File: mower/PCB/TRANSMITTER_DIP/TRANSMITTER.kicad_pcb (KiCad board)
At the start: 2 copper layers, 55 x 41.6 mm, 14 parts, among them J1 BOT POWER, J2 POWER IN, J3 SHUNT, J4 COIL OUT, J5 COIL POWER IN, Q1 IRF3205, U1 LM358, U4 LM555xN

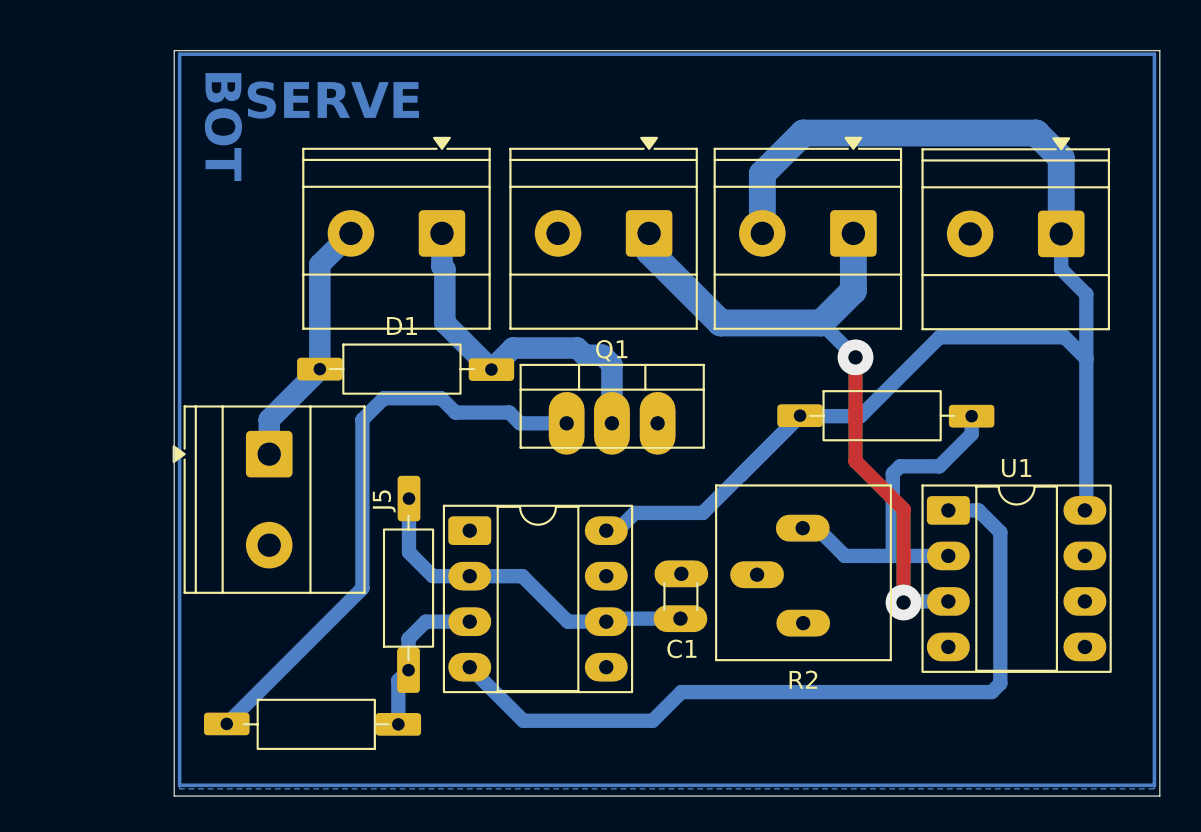
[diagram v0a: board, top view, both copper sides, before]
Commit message: .
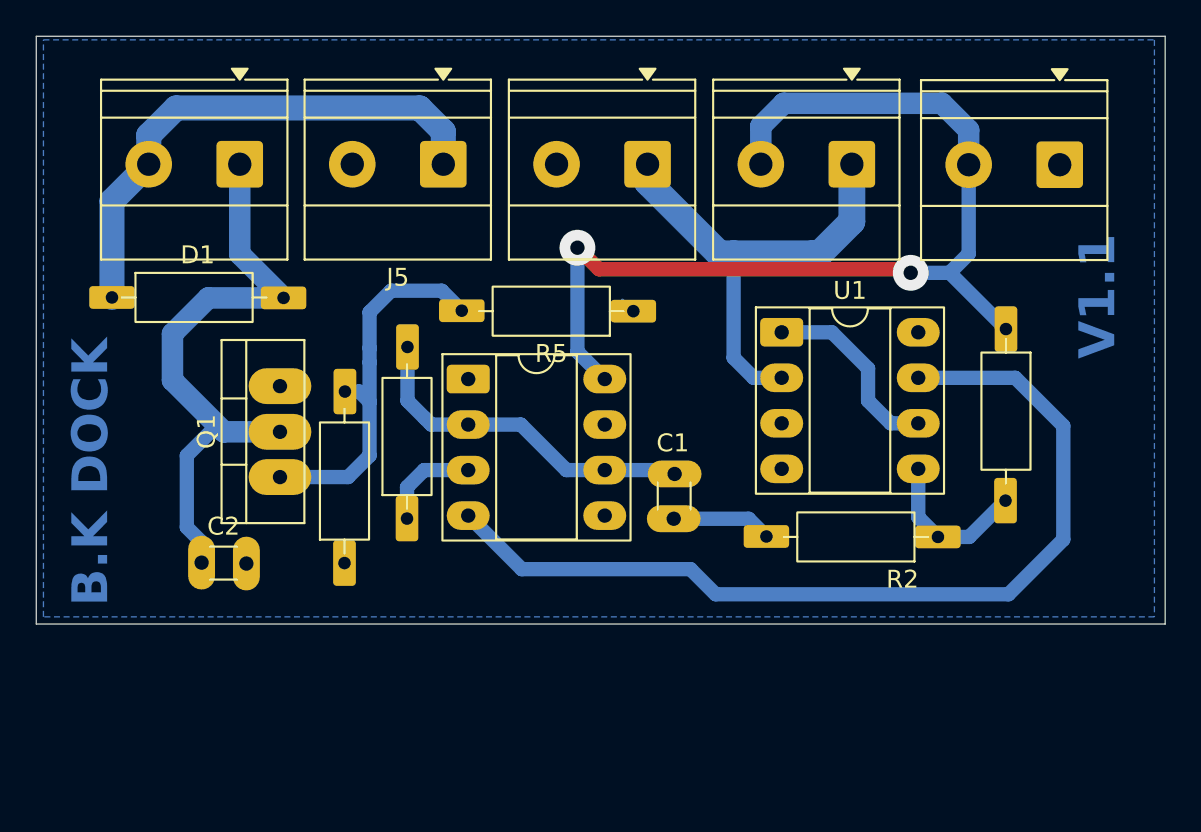
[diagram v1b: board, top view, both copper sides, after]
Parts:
- added C2: 100nF, IMRANS_LIBRARY:C_Disc_D3.0mm_W1.6mm_P2.50mm, F.Cu at (104.0, 63.6)
- added R5: 1K, IMRANS_LIBRARY:R_Axial_DIN0207_L6.3mm_D2.5mm_P10.16mm_Horizontal_2, F.Cu at (128.6, 49.5)
- D1: value 1N5819 -> 1N4007
- R1: value 10k -> 10K
- R2: value 10k -> 10K; footprint IMRANS_LIBRARY:Potentiometer_Bourns_3386P_Vertical -> IMRANS_LIBRARY:R_Axial_DIN0207_L6.3mm_D2.5mm_P10.16mm_Horizontal_2
- moved J5 18.9 mm to (117.5, 41.3), turned to 180 degrees
- moved Q1 16.3 mm to (108.4, 58.8), turned to 90 degrees
- moved U1 13.6 mm to (136.4, 50.7)
- moved R1 13.1 mm to (148.9, 50.0), turned to -90 degrees
- moved D1 12.3 mm to (98.5, 48.8)
- moved J4 11.9 mm to (106.2, 41.3)
- moved R4 9.19 mm to (112.0, 64.1), turned to 90 degrees
- moved R3 8.46 mm to (115.5, 61.6)
- moved U4 8.46 mm to (118.9, 53.3)
- moved C1 8.13 mm to (130.4, 58.6), turned to -90 degrees
- moved R2 8.04 mm to (145.6, 62.1)
- moved J1 3.86 mm to (128.9, 41.3)
- moved J2 3.86 mm to (151.9, 41.4)
- moved J3 3.86 mm to (140.3, 41.3)
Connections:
- J2 pad 1: VCC -> GND
- J2 pad 2: GND -> VCC
- R1 pad 2: Net-(U1A--) -> Net-(U1B-+)
- R2 pad 1: Net-(U1A--) -> Net-(U1B-+)
- U1 pad 1: Net-(U4-R) -> Net-(U1B--)
- U1 pad 2: Net-(U1A--) -> Net-(J1-Pin_1)
- U1 pad 3: Net-(J1-Pin_1) -> GND
- U1 pad 4: GND -> unconnected-(U1C-V--Pad4)
- U1 pad 5: (no net) -> Net-(U1B-+)
- U1 pad 6: (no net) -> Net-(U1B--)
- U1 pad 7: (no net) -> Net-(U4-R)
- U1 pad 8: VCC -> unconnected-(U1C-V+-Pad8)
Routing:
- net VCC: track 79.1 -> 57.0 mm, vias 0 -> 2
- net Net-(U1A--): track 18.9 -> 0.00 mm
- net VCOIL: track 14.2 -> 29.3 mm
- net Net-(D1-A): track 20.3 -> 34.2 mm
- net Net-(Q1-G): track 34.0 -> 21.2 mm
- net Net-(J1-Pin_1): track 38.0 -> 27.0 mm, vias 2 -> 0
- net Net-(U1B--): track 0.00 -> 10.8 mm
- net Net-(U1B-+): track 0.00 -> 8.86 mm
- net Net-(U4-R): track 43.6 -> 51.8 mm
- net GND: track 0.00 -> 7.19 mm
- net Net-(U4-Q): track 8.82 -> 5.56 mm
- net Net-(U4-THR): track 20.6 -> 19.8 mm
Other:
- board size 55 x 41.6 mm -> 63 x 32.8 mm
- board text added: "B.K DOCK"
- board text added: "V1.1"
- board text removed: "BOT"
- board text removed: "SERVE"
